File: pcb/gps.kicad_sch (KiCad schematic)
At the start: 3 parts, among them U3 MAX-M10S

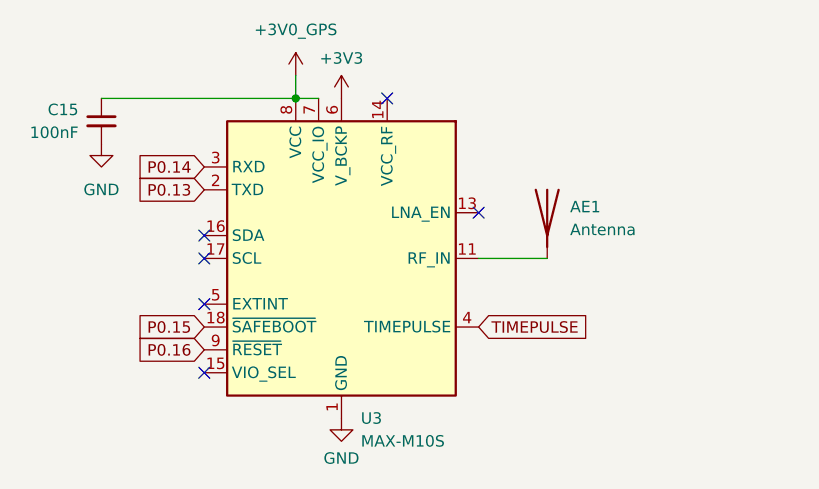
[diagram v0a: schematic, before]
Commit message: mogus
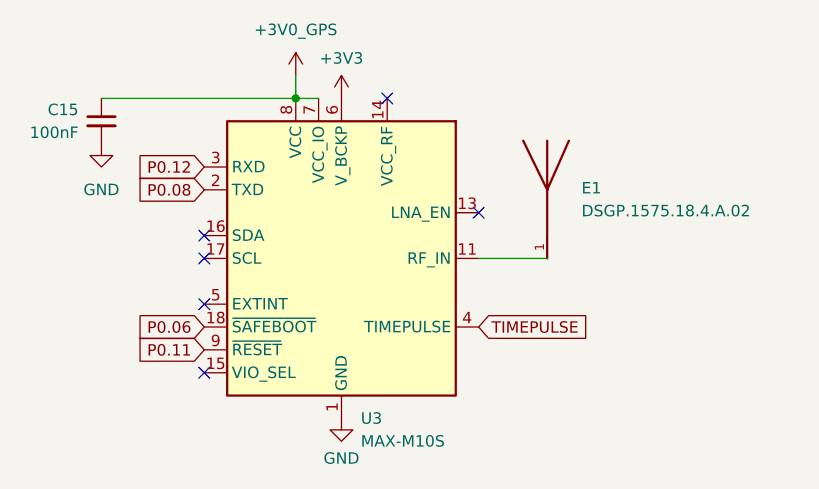
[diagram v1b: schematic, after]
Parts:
- removed AE1: Antenna, JLCImport:KH-GPS181804-WY, symbol Device:Antenna
- added E1: DSGP.1575.18.4.A.02, antrenna:XCVR_DSGP.1575.18.4.A.02, symbol antenna:DSGP.1575.18.4.A.02
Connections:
- net at U3.11 (RF_IN): now also E1.1
- net P0.13 renamed P0.08
- net P0.14 renamed P0.12
- net P0.15 renamed P0.06
- net P0.16 renamed P0.11

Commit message: almost done?
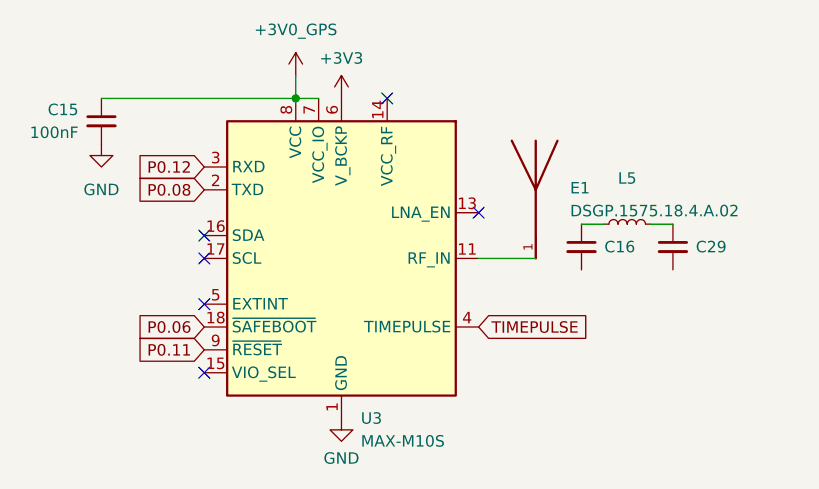
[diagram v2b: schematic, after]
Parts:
- added C16, C29: ?, symbol Device:C_Small
- added L5: ?, Inductor_SMD:L_0603_1608Metric_Pad1.05x0.95mm_HandSolder, symbol Device:L_Small
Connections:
- new net: C16.1, L5.1
- new net: C29.1, L5.2
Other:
- moved on the sheet: E1
